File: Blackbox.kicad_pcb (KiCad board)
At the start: 2 copper layers, 77 x 34.5 mm, 36 parts, among them CN1 SM04B-SRSS-TB (LF)(SN), U1 SN65HVD232DR, U2 STM32G0B1CCT6, U3 BM06B-SRSS-TB(LF)(SN), X2 DSX321G-48M

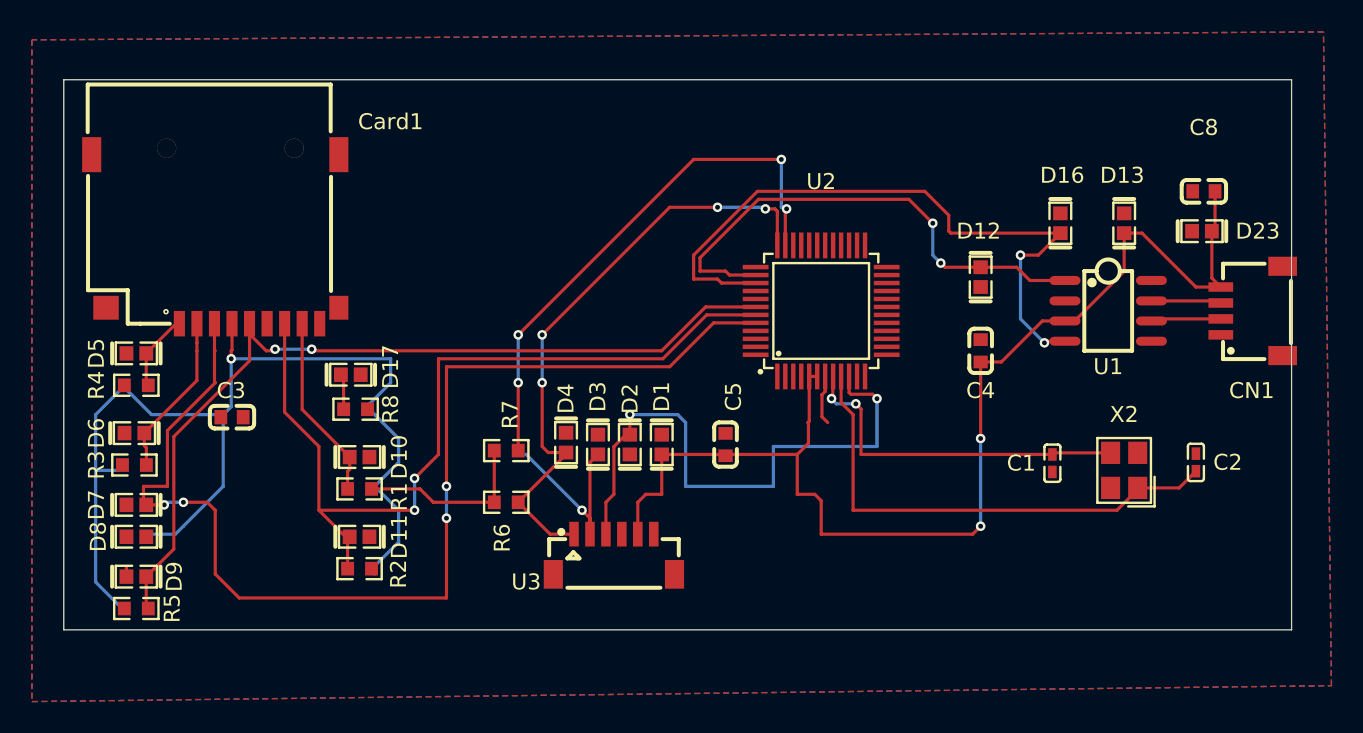
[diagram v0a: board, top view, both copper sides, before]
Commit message: updated pcb
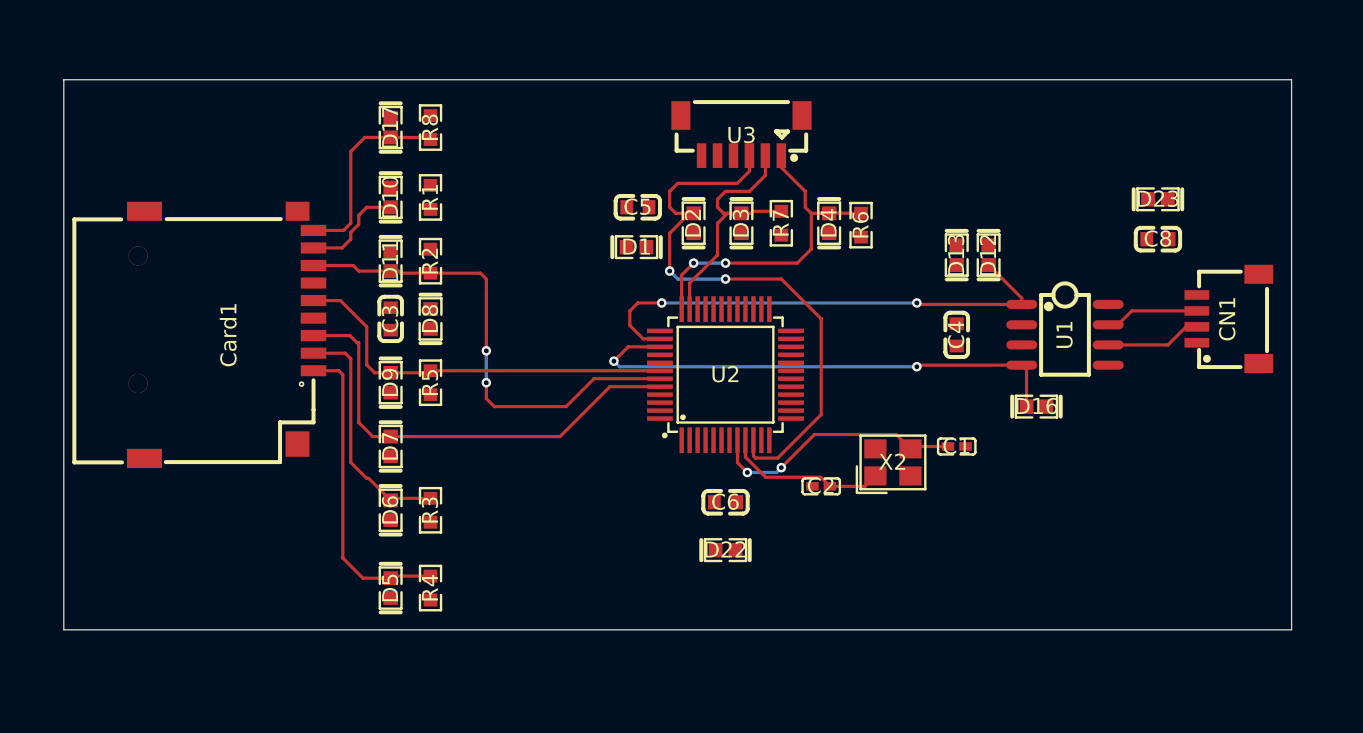
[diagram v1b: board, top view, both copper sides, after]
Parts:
- added C6: 100nF, EasyEDA:C0603, F.Cu at (144.0, 113.0)
- added D22: 0603ESDA-05N, EasyEDA:D0603-BI, F.Cu at (144.0, 116.0)
- moved R6 28.2 mm to (152.5, 95.6), turned to 90 degrees
- moved U3 27.5 mm to (145.0, 90.0), turned to 180 degrees
- moved C2 23.5 mm to (150.0, 112.0), turned to 0 degrees
- moved R5 23.3 mm to (125.5, 105.5), turned to 90 degrees
- moved D8 23.0 mm to (125.5, 101.5), turned to -90 degrees
- moved R4 22.4 mm to (125.5, 118.4), turned to 90 degrees
- moved R7 22.4 mm to (147.5, 95.5), turned to 90 degrees
- moved D5 21.7 mm to (123.0, 118.4), turned to 90 degrees
- moved D4 21.5 mm to (150.5, 95.5), turned to 90 degrees
- moved D9 20.1 mm to (123.0, 105.5), turned to 90 degrees
- moved R2 19.8 mm to (125.5, 97.9), turned to -90 degrees
- moved R1 18.8 mm to (125.5, 93.9), turned to -90 degrees
- moved R3 18.8 mm to (125.5, 113.5), turned to 90 degrees
- moved R8 18.3 mm to (125.5, 89.5), turned to -90 degrees
- moved D11 17.4 mm to (123.0, 97.9), turned to 90 degrees
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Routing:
- net VDD: track 154.4 -> 0.00 mm, vias 3 -> 0
- net CMD: track 73.0 -> 28.6 mm, vias 4 -> 0
- net CLK: track 55.0 -> 25.1 mm, vias 2 -> 0
- net SWDIO: track 46.4 -> 16.6 mm, vias 5 -> 0
- net Dat0: track 54.4 -> 30.5 mm
- net Net-(U2-PF1-OSC_OUT): track 31.3 -> 10.2 mm
- net SWCLK: track 37.7 -> 20.7 mm, vias 4 -> 2
- net Dat2: track 4.91 -> 19.5 mm
- net RX: track 42.3 -> 31.8 mm
- net CD: track 2.23 -> 12.4 mm
- net Net-(U2-PF0-OSC_IN): track 22.1 -> 16.3 mm
- net Dat1: track 11.7 -> 6.48 mm
- net Dat3: track 10.3 -> 15.0 mm
- net GND: track 3.96 -> 0.00 mm
- net Net-(U1-CANL): track 4.40 -> 6.03 mm
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- added copper zone on In1.Cu, net VDD
- removed copper zone on B.Cu, net GND
- removed copper zone on F.Cu, net GND
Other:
- copper layers 2 -> 4
